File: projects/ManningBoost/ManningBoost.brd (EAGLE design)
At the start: 30.1 x 24.1 mm, 27 parts, among them Q1 2N3904

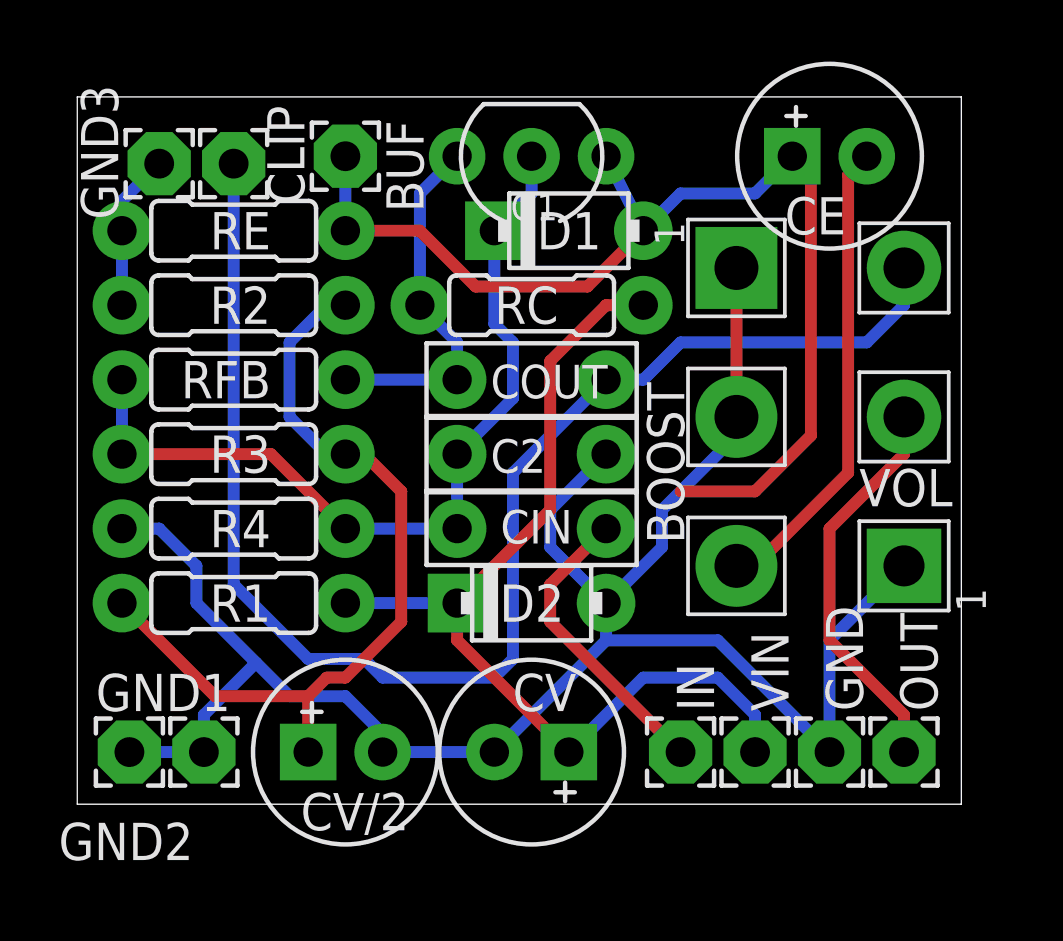
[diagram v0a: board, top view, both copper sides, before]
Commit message: Final project updates. Ready to send to oshpark.
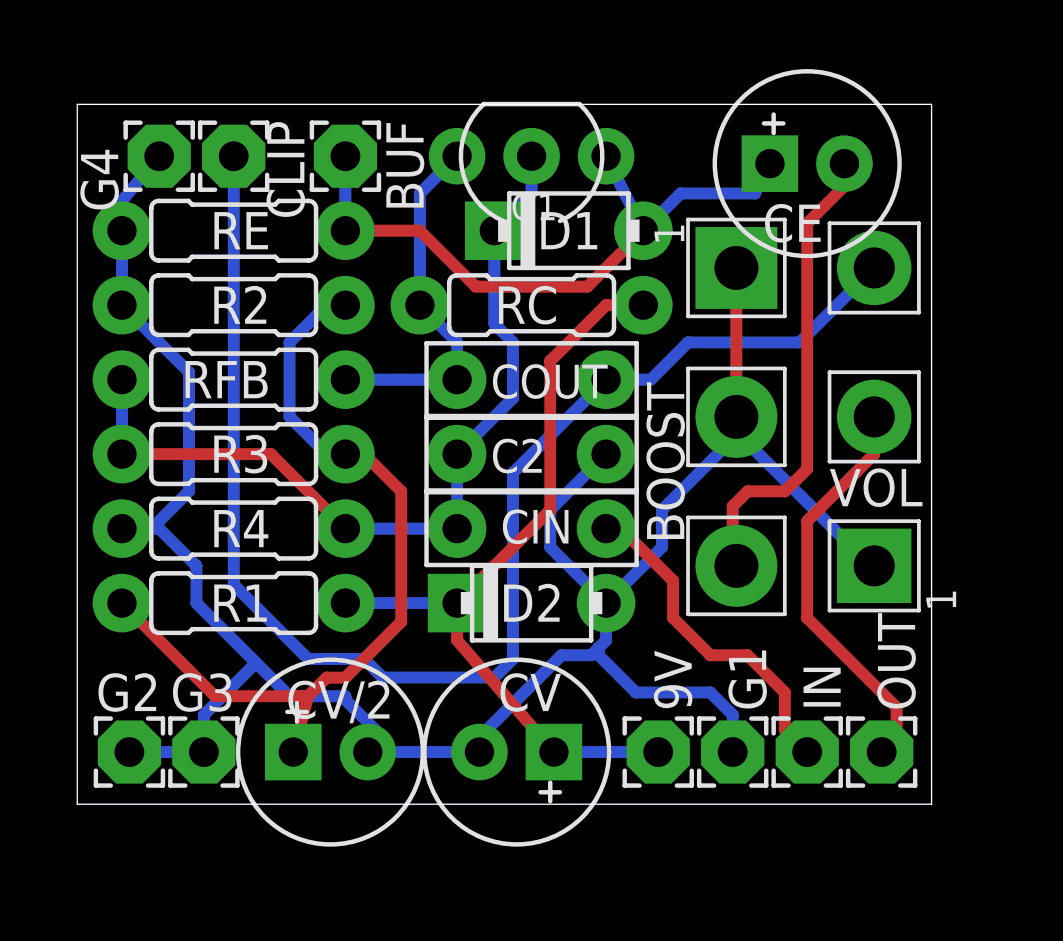
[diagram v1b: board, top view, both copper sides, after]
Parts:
- removed GND, GND3, VIN: (no value), wirepad:2,15/1,0
- added 9V, G1, G4: (no value), wirepad:2,15/1,0
- moved IN 4.32 mm to (24.9, 1.78)
- moved VOL 1.02 mm to (27.2, 13.2)
- moved CE 0.80 mm to (24.9, 21.8)
- moved OUT 0.76 mm to (27.4, 1.78)
- moved CV/2 0.51 mm to (8.64, 1.78)
- moved CV 0.51 mm to (15.0, 1.78)
- moved CLIP 0.25 mm to (5.33, 22.1)
- renumbered GND1 to G2, GND2 to G3
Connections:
- net $3: now also G1.1, G4.1; no longer GND.1, GND3.1
- net N$1: now also 9V.1; no longer VIN.1
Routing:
- net N$7: track 38.3 -> 22.6 mm
- net $3: track 71.8 -> 79.9 mm
- net N$1: track 33.2 -> 27.2 mm
- net N$12: track 48.8 -> 47.3 mm
- net N$9: track 10.3 -> 11.5 mm
- net N$5: track 16.2 -> 17.2 mm
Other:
- board size 30.1 x 24.1 mm -> 29.1 x 23.9 mm
- board text added: "GJCAMANN(C)2014"
- board text added: "ManningBoost"
- board text added: "V1.0"
